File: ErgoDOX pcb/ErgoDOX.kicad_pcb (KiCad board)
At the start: 2 copper layers, 182.8 x 158.9 mm, 77 parts, among them J1 USB, J2 3.5mm, J3 JMP, J4 JMP, SW0:10 SW0:3, SW0:11 SW0:2, SW0:12 SW0:1, SW0:7 SW0:6, SW0:8 SW0:5, SW0:9 SW0:4, SW1:10 SW1:3, SW1:11 SW1:2, SW1:12 SW1:1, SW1:13 SW1:0, SW1:9 SW1:4, SW2:10 SW2:3, SW2:11 SW2:2, SW2:12 SW2:1, SW2:13 SW2:0, SW2:7 SW2:6, SW2:8 SW2:5, SW2:9 SW2:4, SW3:10 SW3:3, SW3:11 SW3:2, SW3:12 SW3:1, SW3:13 SW3:0, SW3:8 SW3:5, SW3:9 SW3:4, SW4:10 SW4:3, SW4:11 SW4:2, SW4:12 SW4:1, SW4:13 SW4:0, SW4:7 SW4:6, SW4:8 SW4:5, SW4:9 SW4:4, SW5:10 SW5:3, SW5:11 SW5:2, SW5:12 SW5:1, SW5:13 SW5:0, SW5:7 SW5:6, SW5:8 SW5:5, SW5:9 SW5:4, U1 TEENSY2.0, U2 MCP23018

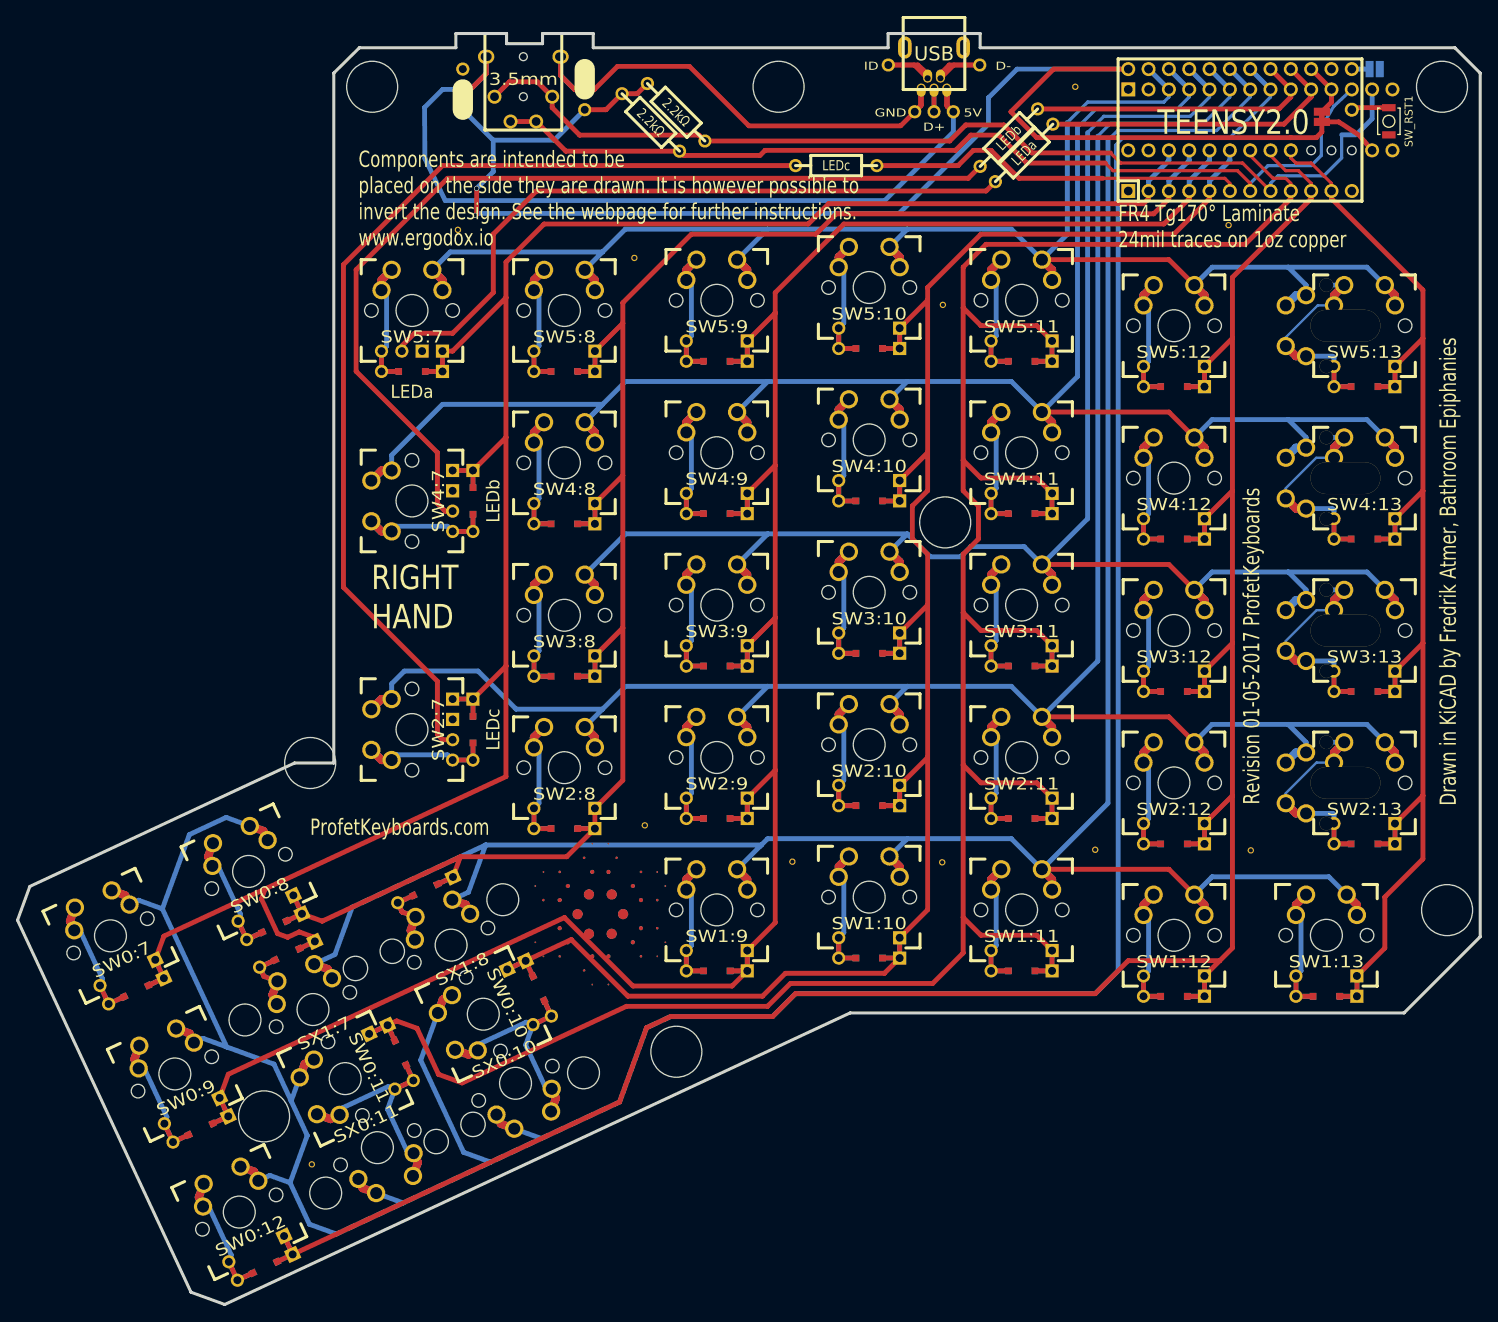
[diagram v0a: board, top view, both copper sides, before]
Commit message: wip
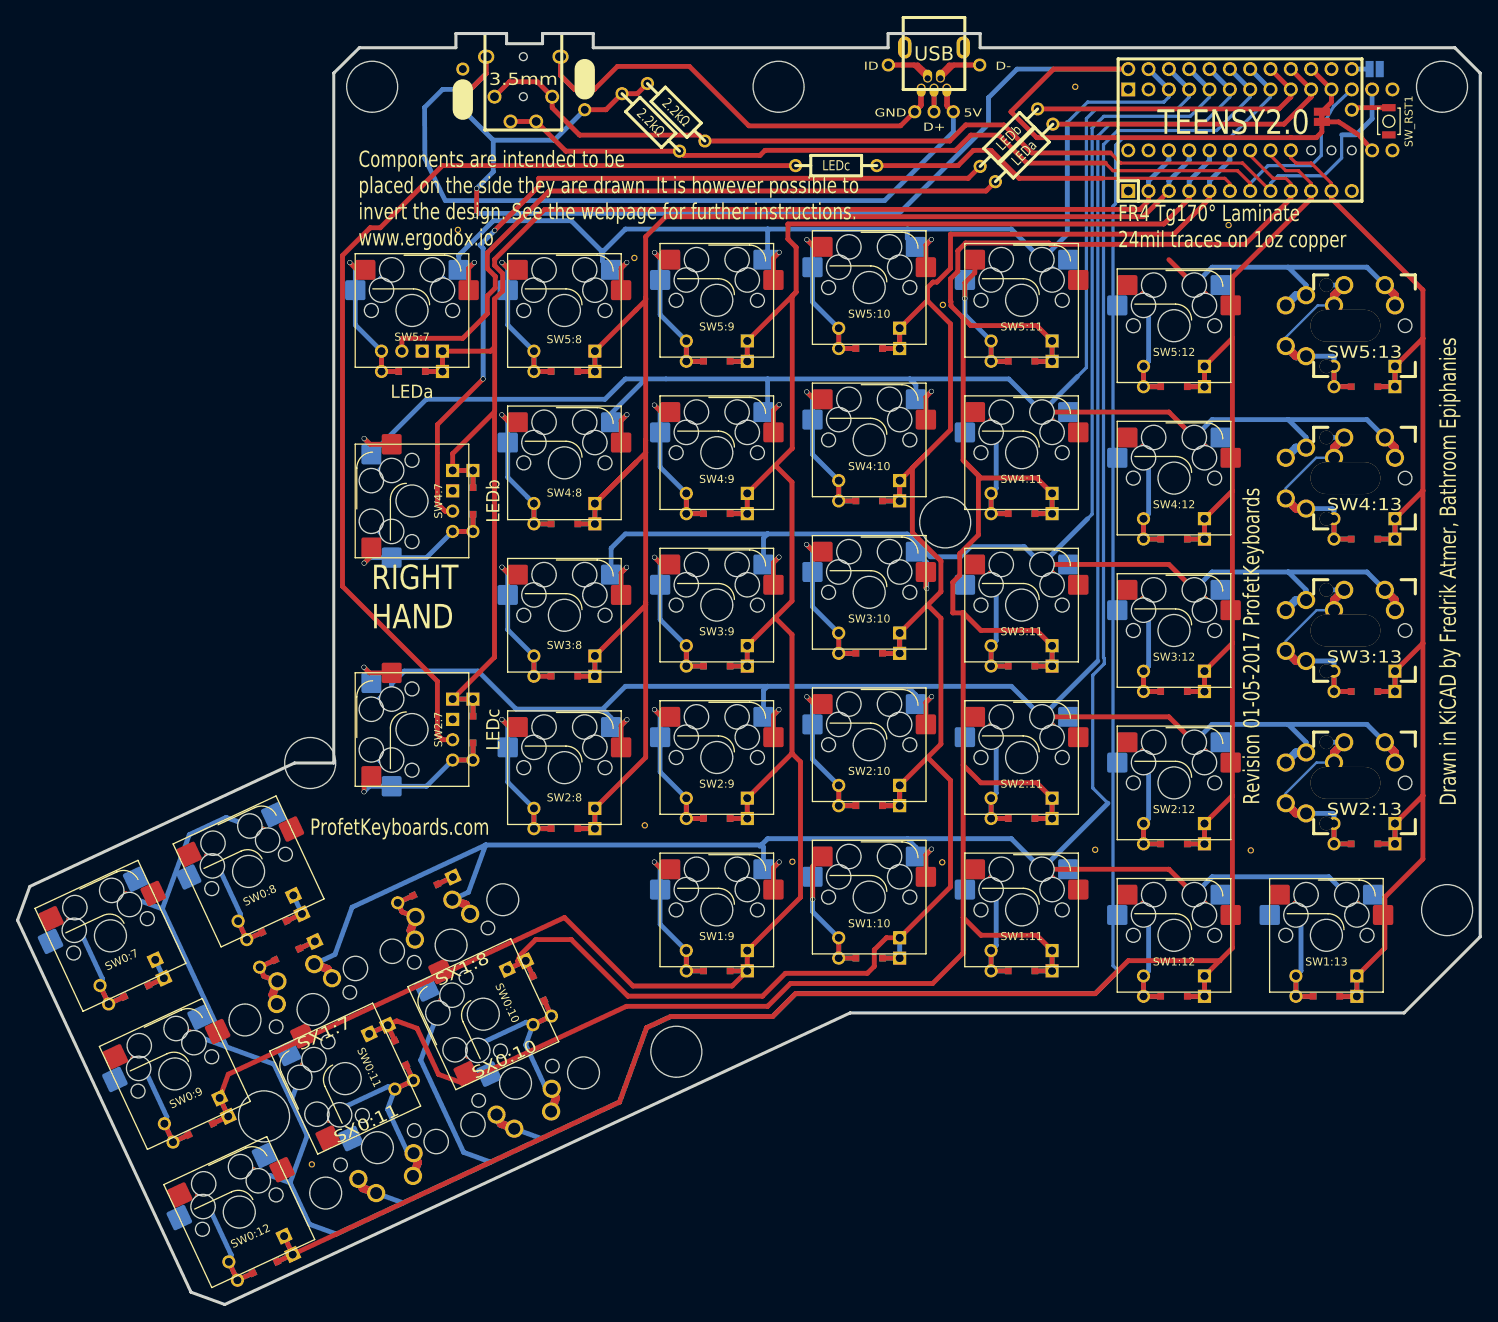
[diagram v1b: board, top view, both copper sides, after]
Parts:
- removed STAR_1: STAR_FRONT, ErgoDOX pcb:STAR
- removed STAR_2: STAR_BACK, ErgoDOX pcb:STAR
- SW0:10, SW0:11, SW0:12, SW0:7, SW0:8, SW0:9, SW1:10, SW1:11, SW1:12, SW1:13, SW1:9, SW2:10, SW2:11, SW2:12, SW2:7, SW2:8, SW2:9, SW3:10, SW3:11, SW3:12, SW3:8, SW3:9, SW4:10, SW4:11, SW4:12, SW4:7, SW4:8, SW4:9, SW5:10, SW5:11, SW5:12, SW5:7, SW5:8, SW5:9: footprint ErgoDOX pcb:MX_FLIP_DIODE -> ErgoDOX pcb:SW_Hotswap_Kailh_MX
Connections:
- SX0:10 pad 1: /ROW0 -> /ROW1
- SX0:11 pad 1: /ROW0 -> /ROW1
- U1 pad 23: /ROW0 -> /ROW1
- U2 pad 8: /ROW0 -> /ROW1
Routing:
- net /ROW1: track 318.2 -> 704.5 mm, vias 0 -> 2
- net /ROW0: track 404.2 -> 18.4 mm
- net /COL6: track 259.5 -> 190.2 mm
- net /ROW5: track 225.1 -> 206.1 mm, vias 0 -> 4
- net /COL5: track 225.8 -> 207.4 mm
- net /COL4: track 274.3 -> 290.3 mm
- net Net-(LED_B1-Pad1): track 119.1 -> 104.3 mm, vias 0 -> 2
- net /COL10: track 233.7 -> 244.6 mm
- net Net-(SW5:7-Pad2): track 19.4 -> 25.0 mm, vias 0 -> 1
- net Net-(SW2:7-Pad2): track 19.4 -> 24.1 mm, vias 0 -> 1
- net Net-(SW4:7-Pad2): track 19.4 -> 24.1 mm, vias 0 -> 1
- net /COL11: track 316.5 -> 320.9 mm
- net /ROW3: track 238.7 -> 234.6 mm, vias 0 -> 3
- net /ROW4: track 257.4 -> 260.8 mm, vias 0 -> 4
- net Net-(LED_A1-Pad1): track 87.6 -> 89.2 mm
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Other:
- net class Default removed
